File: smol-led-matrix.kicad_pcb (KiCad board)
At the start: 4 copper layers, 46.4 x 20.4 mm, 320 parts, among them J1 USB_C_Receptacle_USB2.0, J2 TagConnect_TC2030_SWD, Q1 FS8205, Q2 AO3401A, SW1 SW_Push, SW2 SW_Push, U1 STM32L433CBTx, U2 TP4054, U3 DW01+G, U4 XC6206P332MR

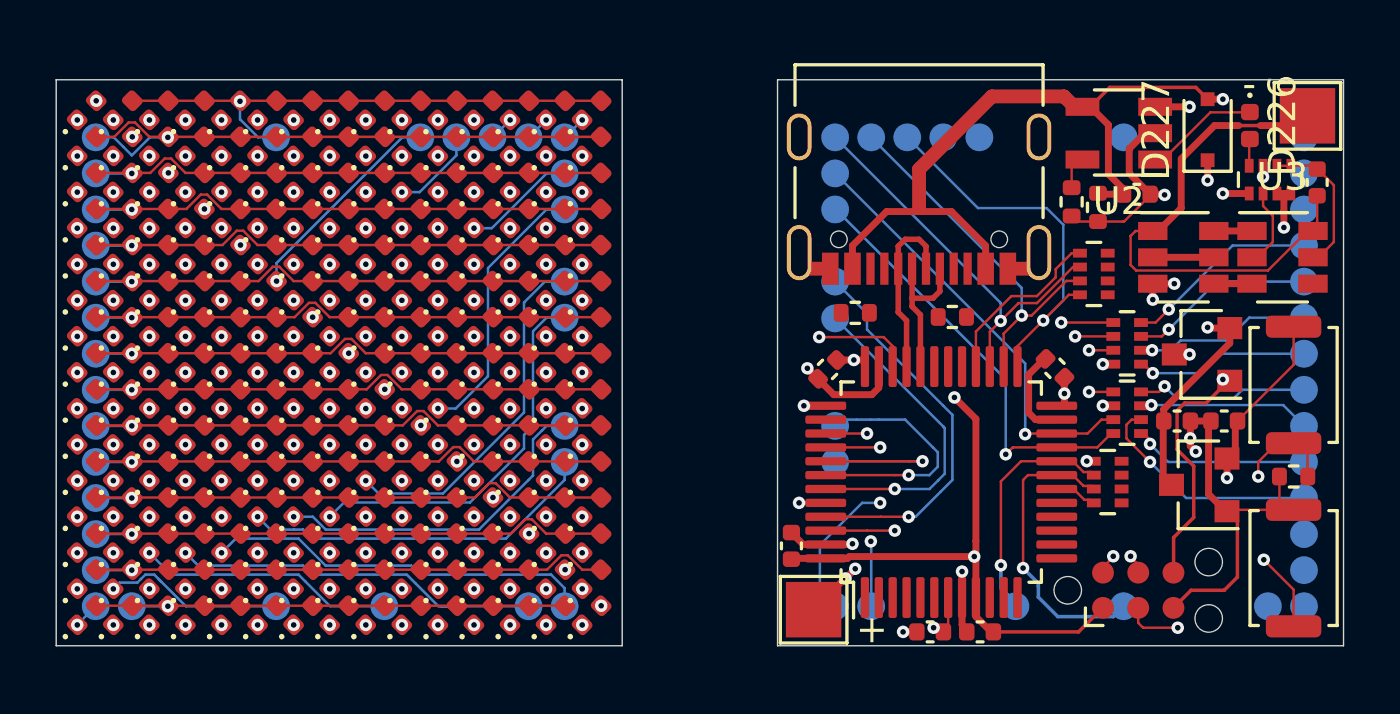
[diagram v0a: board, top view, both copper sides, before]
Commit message: Finish control board layout
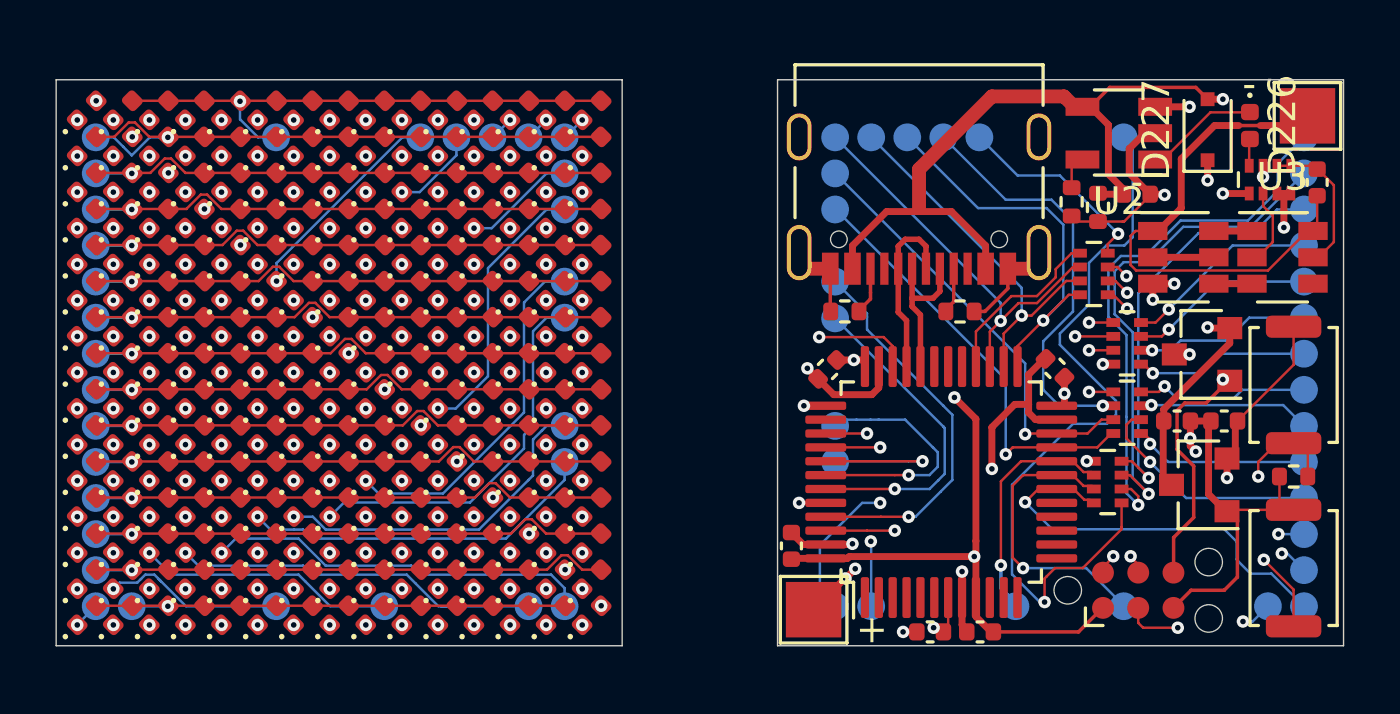
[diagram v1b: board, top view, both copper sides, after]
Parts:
- moved R4 0.38 mm to (128.0, 105.9)
- moved R3 0.34 mm to (132.2, 105.9)
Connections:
- net Net-(R5-Pad2) renamed /BOOT0
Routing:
- net /A0: track 19.1 -> 46.6 mm, vias 1 -> 2
- net /A1: track 21.8 -> 41.3 mm, vias 1 -> 2
- net /A2: track 19.9 -> 38.0 mm, vias 1 -> 2
- net /A14: track 18.2 -> 35.7 mm, vias 1 -> 3
- net /A13: track 19.9 -> 36.6 mm, vias 1 -> 3
- net /A3: track 19.9 -> 35.2 mm, vias 1 -> 2
- net /K9: track 33.6 -> 48.4 mm
- net /K0: track 21.1 -> 34.4 mm, vias 15 -> 16
- net /A12: track 19.9 -> 32.6 mm, vias 1 -> 3
- net /A15: track 40.0 -> 47.3 mm, vias 15 -> 16
- net GND: track 38.0 -> 45.2 mm, vias 10 -> 11
- net Net-(J1-PadB5): track 0.00 -> 1.72 mm
- net Net-(J1-PadA5): track 0.00 -> 1.63 mm
